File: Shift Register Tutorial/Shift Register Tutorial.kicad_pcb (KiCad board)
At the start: 2 copper layers, 134.6 x 162.6 mm, 58 parts, among them J101 USB_A, Q201 2N3904, Q301 2N3904, Q401 2N3904, SW201 SW_Push, SW301 SW_Push, SW401 SW_Push, U101 74164, U102 74164

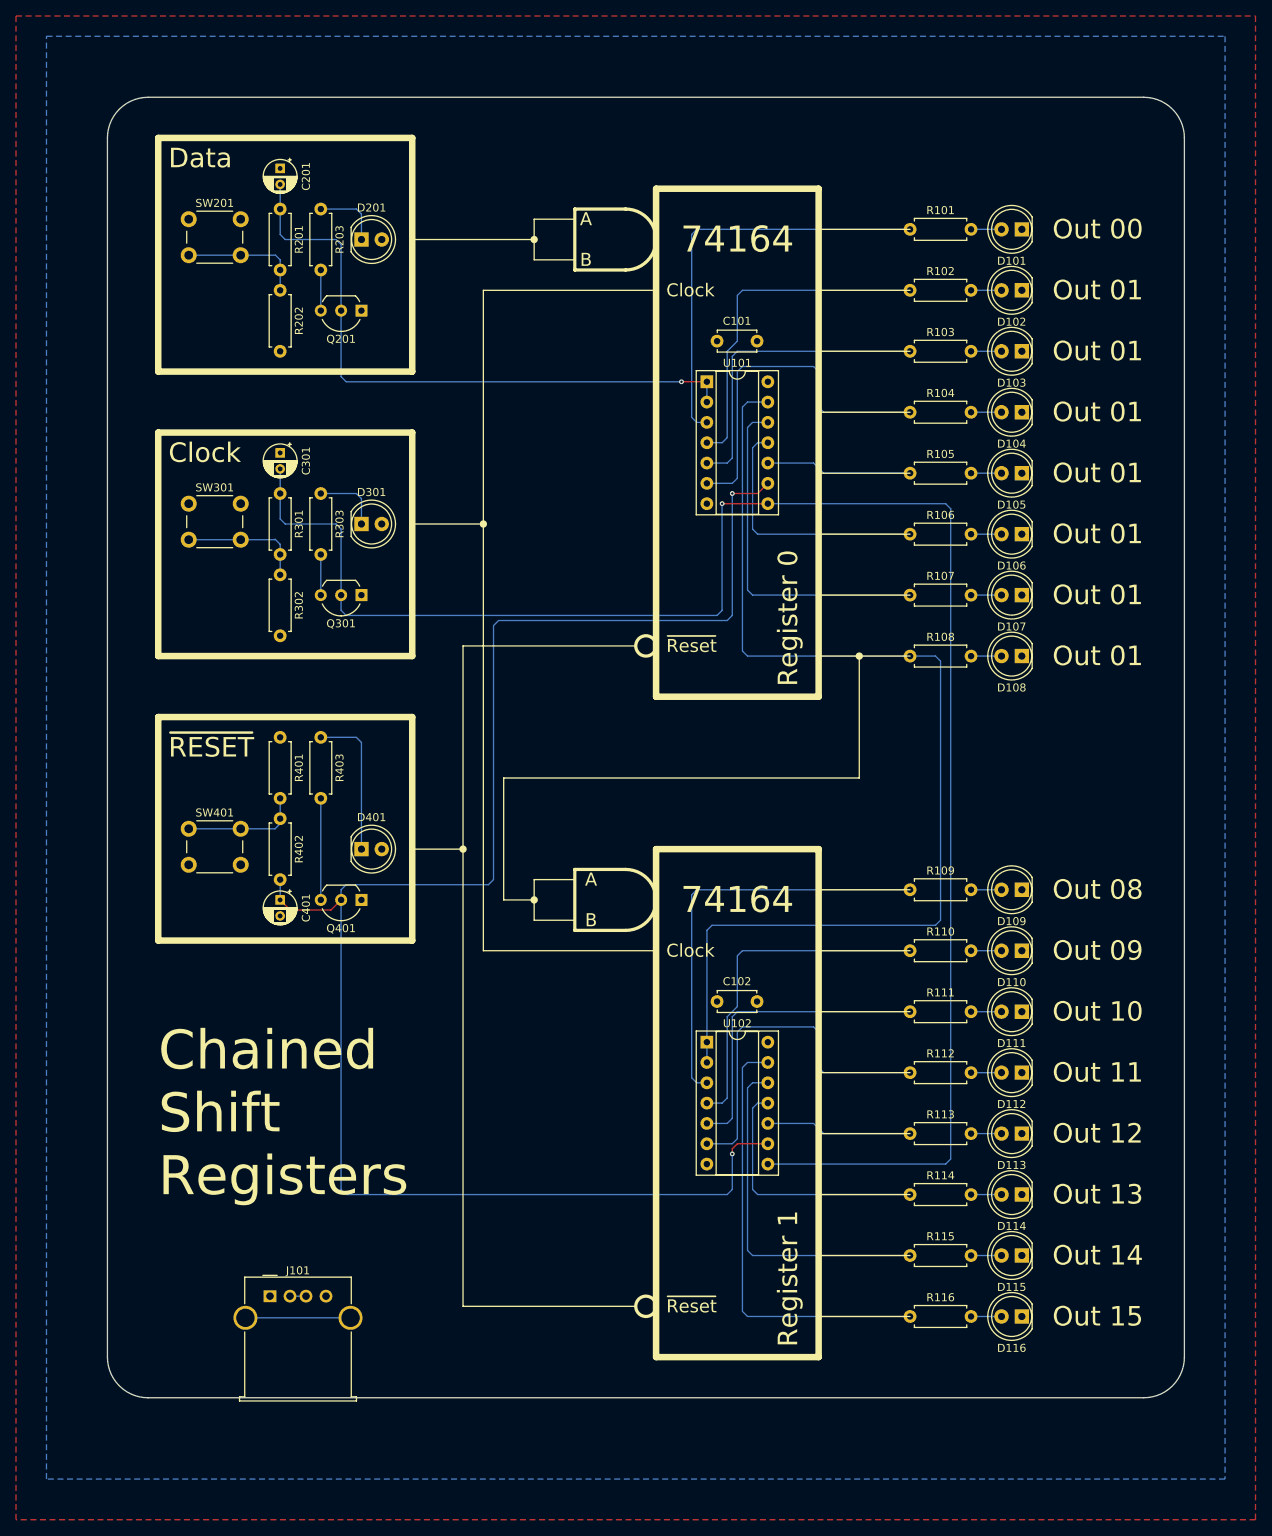
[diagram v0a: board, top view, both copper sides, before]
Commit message: Final tweaks
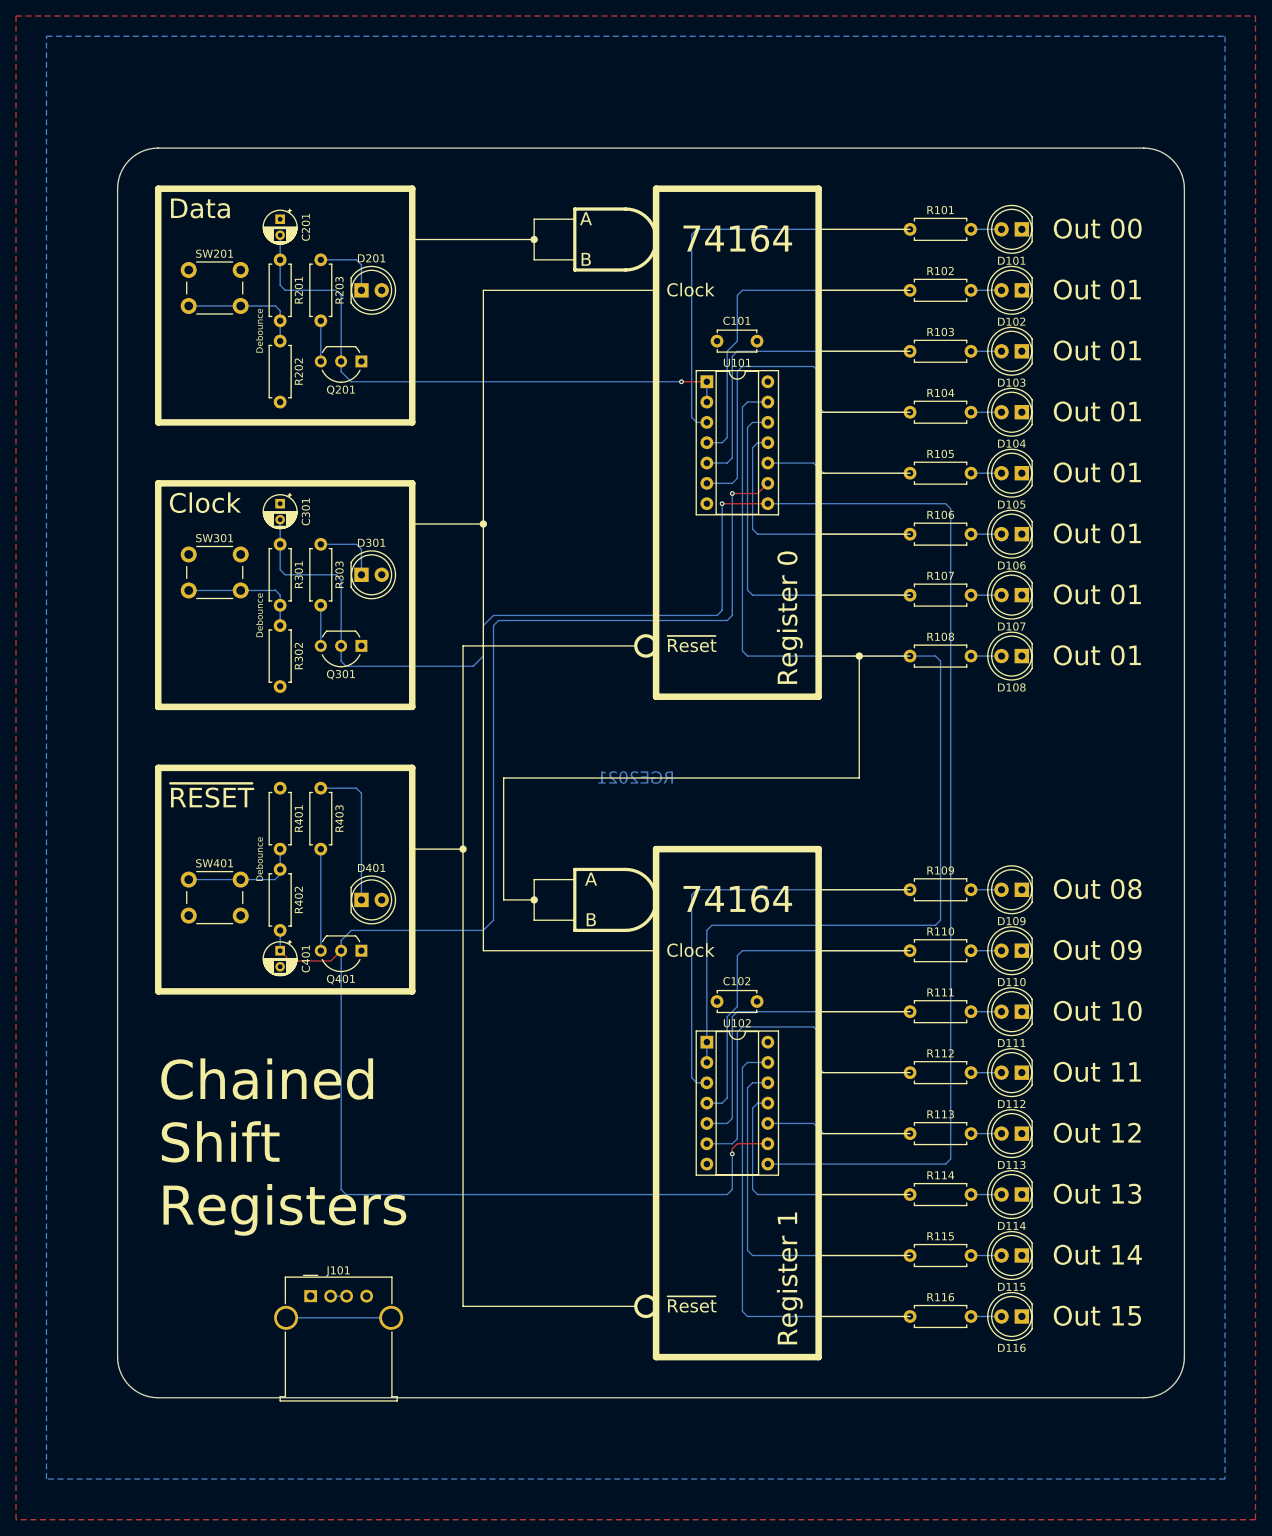
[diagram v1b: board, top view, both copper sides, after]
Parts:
- moved C201 6.35 mm to (-57.1, -52.1)
- moved D201 6.35 mm to (-47.0, -43.2)
- moved D401 6.35 mm to (-47.0, 33.0)
- moved Q201 6.35 mm to (-47.0, -34.3)
- moved R201 6.35 mm to (-57.1, -47.0)
- moved R202 6.35 mm to (-57.1, -36.8)
- moved R203 6.35 mm to (-52.1, -47.0)
- moved R301 6.35 mm to (-57.1, -11.4)
- moved R303 6.35 mm to (-52.1, -11.4)
- moved R401 6.35 mm to (-57.1, 19.1)
- moved R402 6.35 mm to (-57.1, 29.2)
- moved R403 6.35 mm to (-52.1, 19.1)
- moved SW201 6.35 mm to (-68.6, -45.7)
- moved SW301 6.35 mm to (-68.6, -10.2)
- moved SW401 6.35 mm to (-68.6, 30.5)
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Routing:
- net /Data/DATA: track 79.4 -> 72.7 mm
- net /Clock/CLOCK: track 219.3 -> 224.2 mm
- net /~RESET/~RESET: track 209.8 -> 209.1 mm
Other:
- board size 134.6 x 162.6 mm -> 133.3 x 156.2 mm
- board text added: "Debounce"
- board text added: "JLCJLCJLCJLC"
- board text added: "RGE2021"
